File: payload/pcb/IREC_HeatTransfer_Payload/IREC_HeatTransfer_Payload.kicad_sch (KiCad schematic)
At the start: 54 parts, among them J1 Screw_Terminal_01x06, J2 XT60PW-M, J3 Screw_Terminal_01x06, J4 POWER, J5 GPIO, J6 SPI, J7 I2C, J9 Serial, M1 Fan_4pin, U1 MAX31855KASA, U2 MAX31855KASA, U3 MAX31855KASA, U4 AP63357, U5 DS18B20, U6 NJM7805SDL1-TE1, U7 DEV-16771, U8 MPXV7002DP

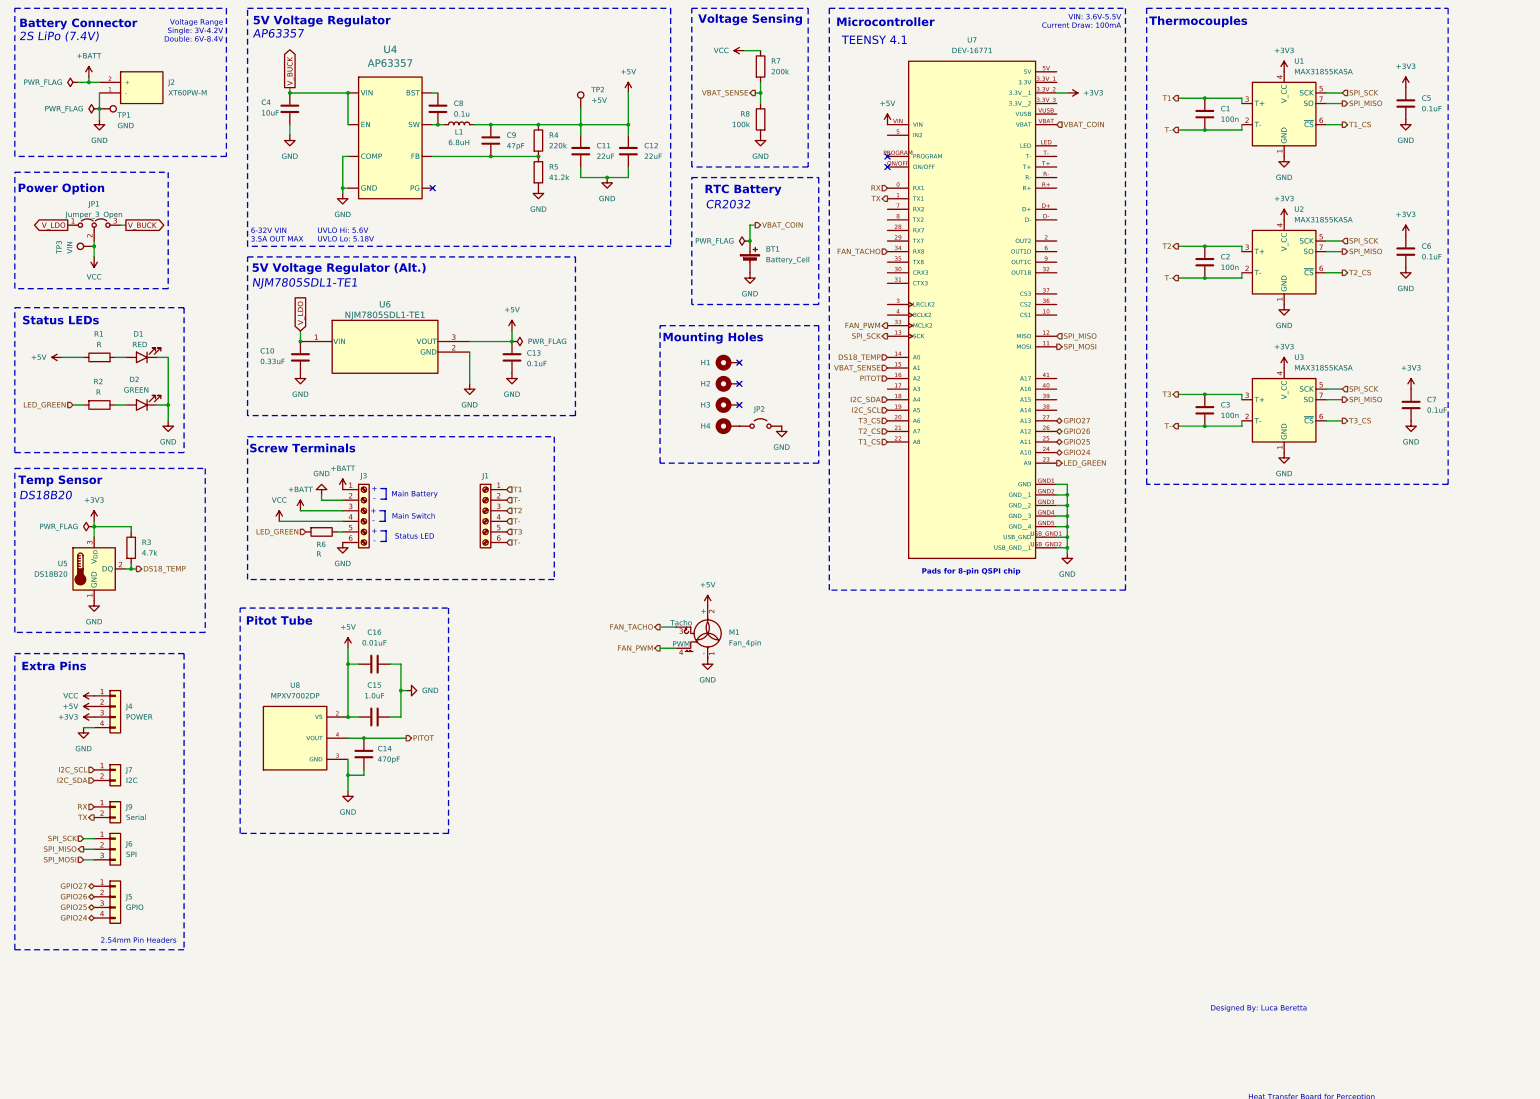
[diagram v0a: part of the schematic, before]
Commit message: upd
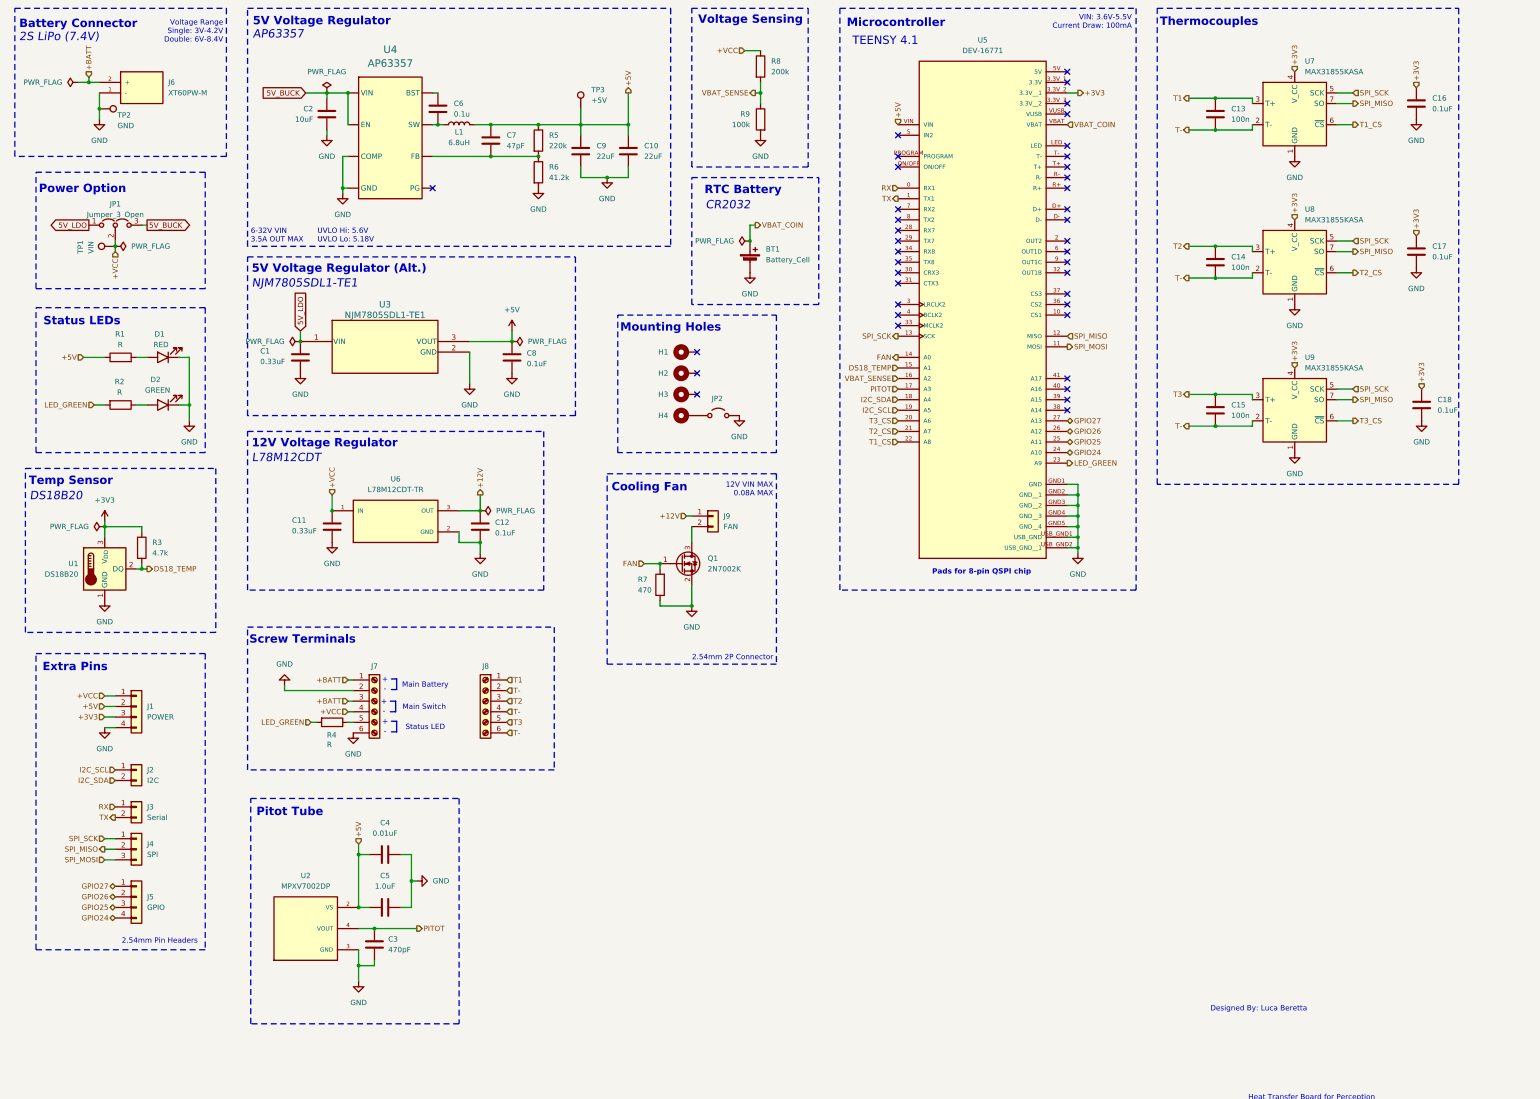
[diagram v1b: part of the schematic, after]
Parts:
- removed M1: Fan_4pin, Connector:FanPinHeader_1x04_P2.54mm_Vertical, symbol Motor:Fan_4pin
- added C11: 0.33uF, Capacitor_SMD:C_0805_2012Metric_Pad1.18x1.45mm_HandSolder, symbol Device:C
- added C12: 0.1uF, Capacitor_SMD:C_0805_2012Metric_Pad1.18x1.45mm_HandSolder, symbol Device:C
- added J9: FAN, Connector_PinHeader_2.54mm:PinHeader_1x02_P2.54mm_Vertical, symbol Connector_Generic:Conn_01x02
- added Q1: 2N7002K, Package_TO_SOT_SMD:SOT-23, symbol Transistor_FET:2N7002K
- added R7: 470, symbol Device:R
- added U6: L78M12CDT-TR, CustomFootprintLib:VREG_L78M12CDT-TR, symbol CustomComponents:L78M12CDT-TR
- renumbered C10 to C1, C12 to C10, C1 to C13, C2 to C14, C3 to C15, C5 to C16, C6 to C17, C7 to C18, C4 to C2, C14 to C3, C16 to C4, C15 to C5, C8 to C6, C9 to C7, C13 to C8, C11 to C9, J4 to J1, J7 to J2, J9 to J3, J6 to J4, J2 to J6, J3 to J7, J1 to J8, R6 to R4, R4 to R5, R5 to R6, R7 to R8, R8 to R9, TP3 to TP1, TP1 to TP2, TP2 to TP3, U5 to U1, U8 to U2, U6 to U3, U7 to U5, U1 to U7, U2 to U8, U3 to U9
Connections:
- net DS18_TEMP: now also U5.15 (A1); no longer U5.14 (A0)
- net GND: now also C11.2, C12.2, Q1.2 (S), R7.1, U6.2 (GND)
- net PITOT: now also U5.17 (A3); no longer U5.16 (A2)
- net VBAT_SENSE: now also U5.16 (A2); no longer U5.15 (A1)
- net FAN_PWM: no longer names the net of U5.33 (MCLK2)
- net FAN_TACHO: no longer names the net of U5.34 (RX8)
- net VCC renamed +VCC
- net +VCC: now also C11.1, U6.1 (IN)
- net V_BUCK renamed 5V_BUCK
- net V_LDO renamed 5V_LDO
- new net: J9.2 (Pin_2), Q1.3 (D)
- new net +12V: C12.1, J9.1 (Pin_1), U6.3 (OUT)
- new net FAN: Q1.1 (G), R7.2, U5.14 (A0)
- no-connect marks 6 -> 40
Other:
- note added: "12V VIN MAX 0.08A MAX"
- note added: "12V Voltage Regulator"
- note added: "2.54mm 2P Connector"
- note added: "Cooling Fan"
- note added: "L78M12CDT"
- moved on the sheet: C13, C14, C15, C16, C17, C18, C2, C3, C4, C5, D1, D2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
